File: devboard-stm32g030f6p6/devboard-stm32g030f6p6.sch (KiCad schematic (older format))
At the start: 23 parts, among them J1 USB_B_Micro, J2 Conn_ARM_JTAG_SWD_10, J3 Pins_Right, J4 Pins_Left, SW1 Reset, U1 STM32G030F6P6, U2 XC6206P332MR, Y1 32MHz

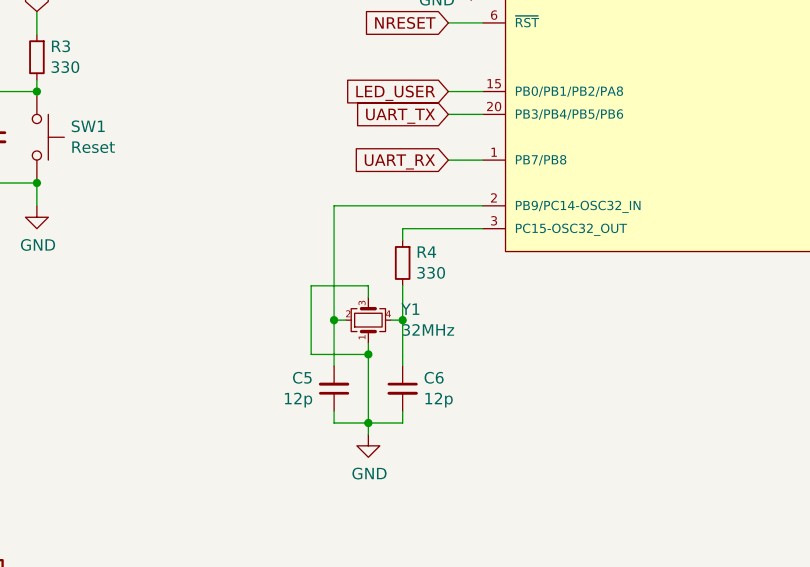
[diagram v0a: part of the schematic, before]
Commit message: Fix oscillator being rotated by 90 degrees
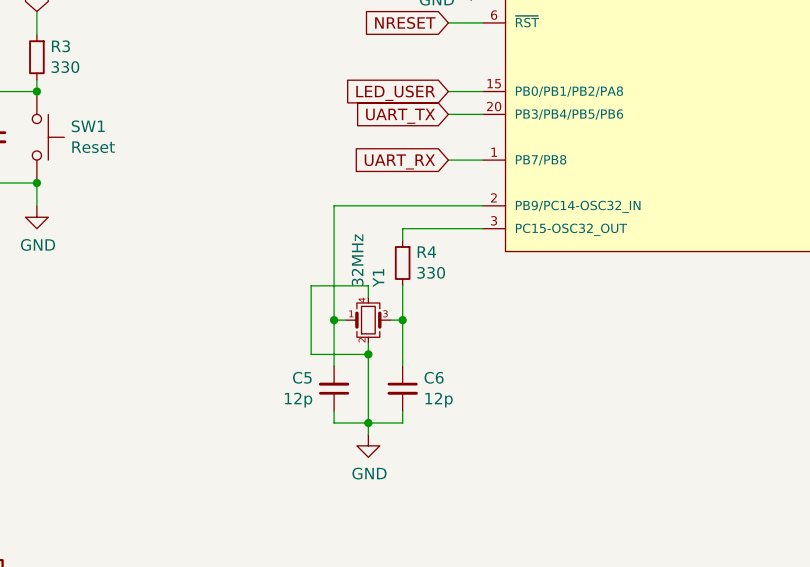
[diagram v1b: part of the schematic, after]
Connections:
- net GND: now also Y1.2, Y1.4; no longer Y1.1, Y1.3
- net at C5.2, U1.2 (PB9/PC14-OSC32_IN): now also Y1.1; no longer Y1.2
- net at C6.1, R4.2: now also Y1.3; no longer Y1.4
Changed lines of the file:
@@
 F 4 "7F32000E12UCG" V 4000 4650 50  0001 C CNN "Part"
 	1    4000 4650
-	0    1    -1   0
+	1    0    0    -1
 $EndComp
 Wire Wire Line

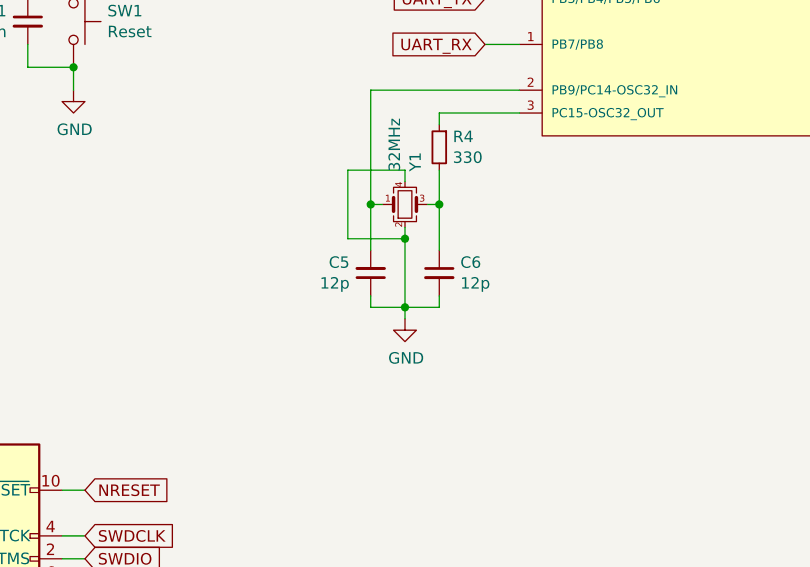
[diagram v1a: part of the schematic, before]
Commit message: Reduce crystal bypass capacitors to 10p, frequency measures too low
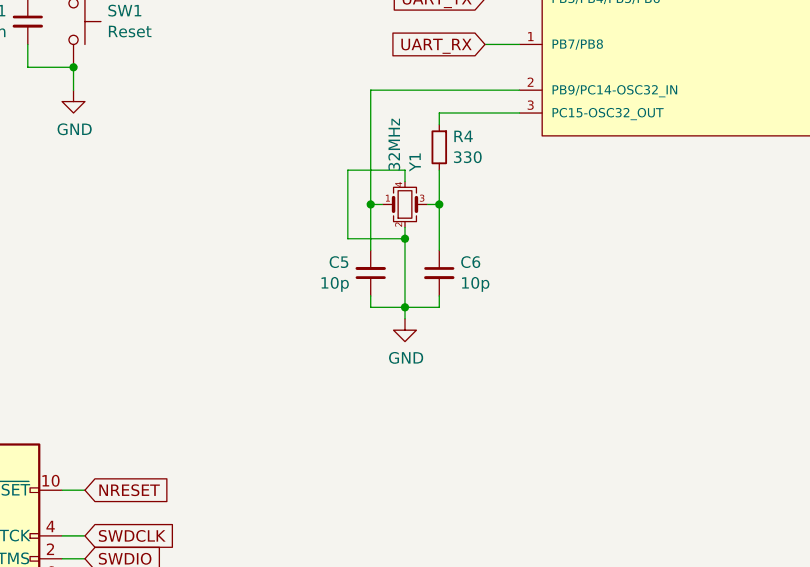
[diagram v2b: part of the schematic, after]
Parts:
- C5, C6: value 12p -> 10p
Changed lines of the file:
@@
 P 3850 4950
 F 0 "C5" H 3758 4904 50  0000 R CNN
-F 1 "12p" H 3758 4995 50  0000 R CNN
+F 1 "10p" H 3758 4995 50  0000 R CNN
 F 2 "Capacitor_SMD:C_0402_1005Metric" H 3850 4950 50  0001 C CNN
 F 3 "~" H 3850 4950 50  0001 C CNN
@@
 P 4150 4950
 F 0 "C6" H 4058 4996 50  0000 R CNN
-F 1 "12p" H 4058 4905 50  0000 R CNN
+F 1 "10p" H 4058 4905 50  0000 R CNN
 F 2 "Capacitor_SMD:C_0402_1005Metric" H 4150 4950 50  0001 C CNN
 F 3 "~" H 4150 4950 50  0001 C CNN

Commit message: Increase crystal bypass caps back up to 12p
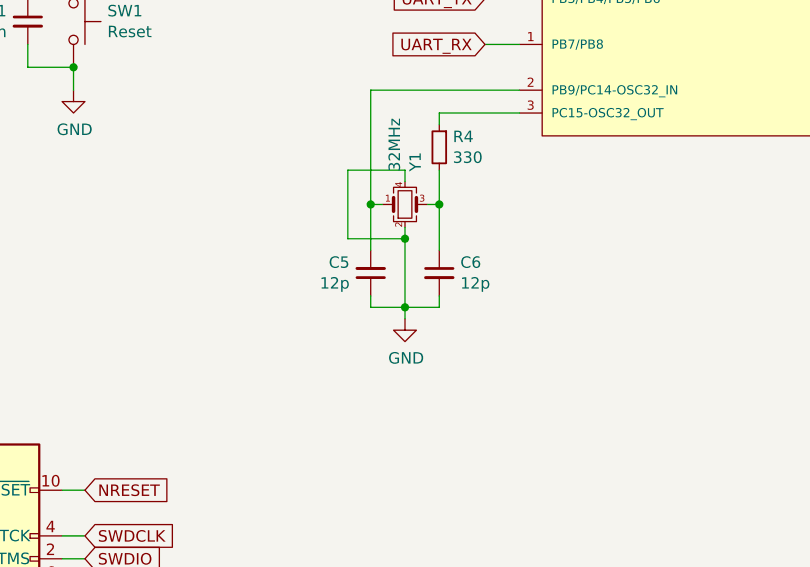
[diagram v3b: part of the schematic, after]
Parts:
- C5, C6: value 10p -> 12p
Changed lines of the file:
@@
 P 3850 4950
 F 0 "C5" H 3758 4904 50  0000 R CNN
-F 1 "10p" H 3758 4995 50  0000 R CNN
+F 1 "12p" H 3758 4995 50  0000 R CNN
 F 2 "Capacitor_SMD:C_0402_1005Metric" H 3850 4950 50  0001 C CNN
 F 3 "~" H 3850 4950 50  0001 C CNN
@@
 P 4150 4950
 F 0 "C6" H 4058 4996 50  0000 R CNN
-F 1 "10p" H 4058 4905 50  0000 R CNN
+F 1 "12p" H 4058 4905 50  0000 R CNN
 F 2 "Capacitor_SMD:C_0402_1005Metric" H 4150 4950 50  0001 C CNN
 F 3 "~" H 4150 4950 50  0001 C CNN
